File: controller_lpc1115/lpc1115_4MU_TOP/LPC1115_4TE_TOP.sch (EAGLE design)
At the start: 102 parts, among them P2 ISP, Q1 BC856, Q2 BCP52, Q3 BC847C, U1 LPC1115FBD48, U2 BD9G101, U3 XO32 12MHz

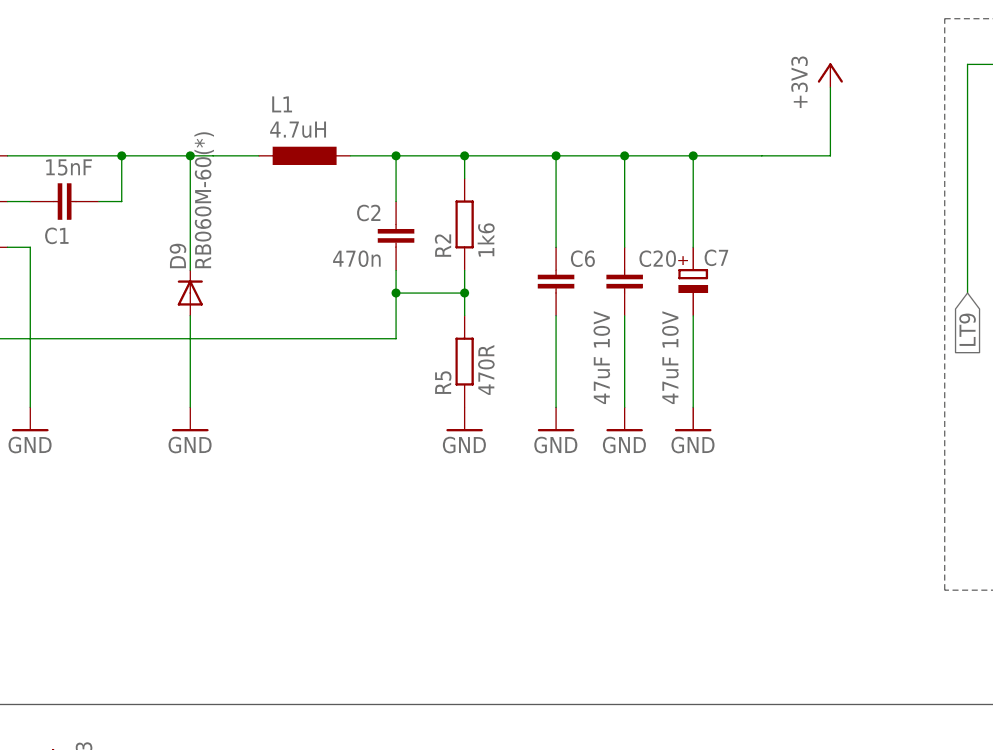
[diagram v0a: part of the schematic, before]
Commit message: [ctrl_4MU_TOP] - v2.0 alpha
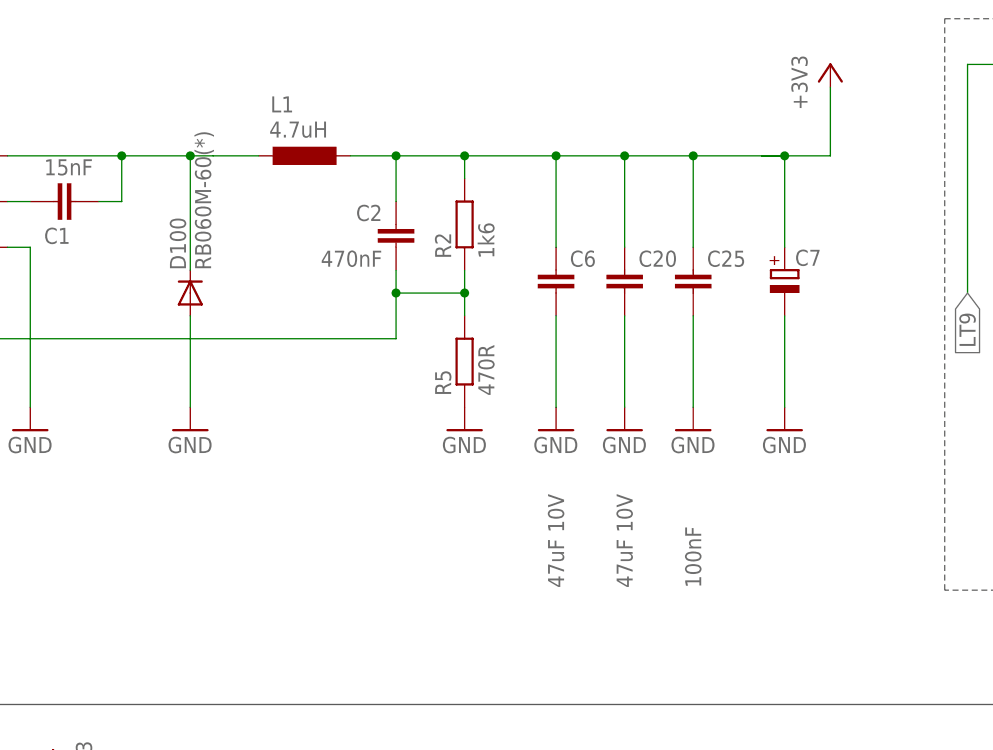
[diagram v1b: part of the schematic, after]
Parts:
- added C25: 100nF, rcl:C-EUC1206
- C2: value 470n -> 470nF
- C20, C6: device rcl:C-EUC1206 -> rcl:C-EUC0805
- renumbered D9 to D100
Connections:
- net +3V3: now also C25.1
- net GND: now also C25.2
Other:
- moved on the sheet: C7
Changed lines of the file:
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@@
 <part name="L1" library="rcl" library_urn="urn:adsk.eagle:library:334" deviceset="L-EU" device="L4532P" package3d_urn="urn:adsk.eagle:package:23484/1" value="4.7uH"/>
 <part name="C4" library="rcl" library_urn="urn:adsk.eagle:library:334" deviceset="C-EU" device="C0805" package3d_urn="urn:adsk.eagle:package:23617/2" value="4.7uF 50V"/>
-<part name="C6" library="rcl" library_urn="urn:adsk.eagle:library:334" deviceset="C-EU" device="C1206" package3d_urn="urn:adsk.eagle:package:23618/2" value="47uF 10V"/>
+<part name="C6" library="rcl" library_urn="urn:adsk.eagle:library:334" deviceset="C-EU" device="C0805" package3d_urn="urn:adsk.eagle:package:23617/2" value="47uF 10V"/>
 <part name="C1" library="rcl" library_urn="urn:adsk.eagle:library:334" deviceset="C-EU" device="C0805" package3d_urn="urn:adsk.eagle:package:23617/2" value="15nF"/>
 <part name="R2" library="rcl" library_urn="urn:adsk.eagle:library:334" deviceset="R-EU_" device="R0805" package3d_urn="urn:adsk.eagle:package:23553/2" value="1k6"/>
 <part name="R5" library="rcl" library_urn="urn:adsk.eagle:library:334" deviceset="R-EU_" device="R0805" package3d_urn="urn:adsk.eagle:package:23553/2" value="470R"/>
-<part name="C2" library="rcl" library_urn="urn:adsk.eagle:library:334" deviceset="C-EU" device="C0805" package3d_urn="urn:adsk.eagle:package:23617/2" value="470n"/>
-<part name="D9" library="diode" deviceset="DIODE-" device="SOD123" value="RB060M-60(*)"/>
+<part name="C2" library="rcl" library_urn="urn:adsk.eagle:library:334" deviceset="C-EU" device="C0805" package3d_urn="urn:adsk.eagle:package:23617/2" value="470nF"/>
+<part name="D100" library="diode" deviceset="DIODE-" device="SOD123" value="RB060M-60(*)"/>
 <part name="+3V35" library="supply1" deviceset="+3V3" device=""/>
 <part name="C13" library="rcl" library_urn="urn:adsk.eagle:library:334" deviceset="C-EU" device="C0805" package3d_urn="urn:adsk.eagle:package:23617/2" value="1uF"/>
@@
 <part name="D15" library="Diode_for_Selfbus-Projects" deviceset="DIODE-ZENER" device="SOD-123" package3d_urn="urn:adsk.eagle:package:40015434/2" value="DDZ9685"/>
 <part name="R1" library="rcl" library_urn="urn:adsk.eagle:library:334" deviceset="R-EU_" device="R2512" package3d_urn="urn:adsk.eagle:package:23545/2" value="24R  2512 1.0W"/>
-<part name="C20" library="rcl" library_urn="urn:adsk.eagle:library:334" deviceset="C-EU" device="C1206" package3d_urn="urn:adsk.eagle:package:23618/2" value="47uF 10V"/>
+<part name="C20" library="rcl" library_urn="urn:adsk.eagle:library:334" deviceset="C-EU" device="C0805" package3d_urn="urn:adsk.eagle:package:23617/2" value="47uF 10V"/>
 <part name="GND4" library="supply1" deviceset="GND" device=""/>
 <part name="C21" library="rcl" library_urn="urn:adsk.eagle:library:334" deviceset="C-EU" device="C0805" package3d_urn="urn:adsk.eagle:package:23617/2" value="100nF"/>
 <part name="C8" library="rcl" library_urn="urn:adsk.eagle:library:334" deviceset="C-EU" device="C0805" package3d_urn="urn:adsk.eagle:package:23617/2" value="100nF"/>
 <part name="C24" library="rcl" library_urn="urn:adsk.eagle:library:334" deviceset="C-EU" device="C0805" package3d_urn="urn:adsk.eagle:package:23617/2" value="1uF"/>
+<part name="C25" library="rcl" library_urn="urn:adsk.eagle:library:334" deviceset="C-EU" device="C1206" package3d_urn="urn:adsk.eagle:package:23618/2" value="100nF"/>
+<part name="GND7" library="supply1" deviceset="GND" device=""/>
 </parts>
 <sheets>
@@
 <instance part="C6" gate="G$1" x="200.66" y="226.06" smashed="yes">
 <attribute name="NAME" x="202.184" y="226.441" size="1.778" layer="95"/>
-<attribute name="VALUE" x="206.629" y="211.074" size="1.778" layer="96" rot="R90"/>
+<attribute name="VALUE" x="201.549" y="190.754" size="1.778" layer="96" rot="R90"/>
 </instance>
 <instance part="C1" gate="G$1" x="147.32" y="233.68" smashed="yes" rot="R270">
@@
 <attribute name="VALUE" x="181.356" y="226.441" size="1.778" layer="96" rot="MR0"/>
 </instance>
-<instance part="D9" gate="G$1" x="160.02" y="223.52" smashed="yes" rot="R90">
+<instance part="D100" gate="G$1" x="160.02" y="223.52" smashed="yes" rot="R90">
 <attribute name="NAME" x="159.5374" y="226.06" size="1.778" layer="95" rot="R90"/>
 <attribute name="VALUE" x="162.3314" y="226.06" size="1.778" layer="96" rot="R90"/>
@@
 <attribute name="SHEET" x="357.505" y="5.08" size="2.54" layer="94"/>
 </instance>
-<instance part="C7" gate="G$1" x="215.9" y="226.06" smashed="yes">
-<attribute name="NAME" x="217.043" y="226.5426" size="1.778" layer="95"/>
-</instance>
-<instance part="GND10" gate="1" x="215.9" y="208.28" smashed="yes">
-<attribute name="VALUE" x="213.36" y="205.74" size="1.778" layer="96"/>
+<instance part="C7" gate="G$1" x="226.06" y="226.06" smashed="yes">
+<attribute name="NAME" x="227.203" y="226.5426" size="1.778" layer="95"/>
+</instance>
+<instance part="GND10" gate="1" x="226.06" y="208.28" smashed="yes">
+<attribute name="VALUE" x="223.52" y="205.74" size="1.778" layer="96"/>
 </instance>
 <instance part="D16" gate="G$1" x="60.96" y="127" smashed="yes" rot="R90">
@@
 <instance part="C20" gate="G$1" x="208.28" y="226.06" smashed="yes">
 <attribute name="NAME" x="209.804" y="226.441" size="1.778" layer="95"/>
-<attribute name="VALUE" x="214.249" y="211.074" size="1.778" layer="96" rot="R90"/>
+<attribute name="VALUE" x="209.169" y="190.754" size="1.778" layer="96" rot="R90"/>
 </instance>
 <instance part="GND4" gate="1" x="208.28" y="208.28" smashed="yes">
@@
 <attribute name="NAME" x="301.244" y="91.821" size="1.778" layer="95"/>
 <attribute name="VALUE" x="301.244" y="86.741" size="1.778" layer="96"/>
+</instance>
+<instance part="C25" gate="G$1" x="215.9" y="226.06" smashed="yes">
+<attribute name="NAME" x="217.424" y="226.441" size="1.778" layer="95"/>
+<attribute name="VALUE" x="216.789" y="190.754" size="1.778" layer="96" rot="R90"/>
+</instance>
+<instance part="GND7" gate="1" x="215.9" y="208.28" smashed="yes">
+<attribute name="VALUE" x="213.36" y="205.74" size="1.778" layer="96"/>
 </instance>
 </instances>
@@
 </segment>
 <segment>
-<pinref part="D9" gate="G$1" pin="A"/>
+<pinref part="D100" gate="G$1" pin="A"/>
 <wire x1="160.02" y1="220.98" x2="160.02" y2="210.82" width="0.1524" layer="91"/>
 <pinref part="GND6" gate="1" pin="GND"/>
@@
 <pinref part="C7" gate="G$1" pin="-"/>
 <pinref part="GND10" gate="1" pin="GND"/>
-<wire x1="215.9" y1="220.98" x2="215.9" y2="210.82" width="0.1524" layer="91"/>
+<wire x1="226.06" y1="220.98" x2="226.06" y2="210.82" width="0.1524" layer="91"/>
 </segment>
 <segment>
@@
 <wire x1="208.28" y1="220.98" x2="208.28" y2="210.82" width="0.1524" layer="91"/>
 <pinref part="GND4" gate="1" pin="GND"/>
+</segment>
+<segment>
+<pinref part="C25" gate="G$1" pin="2"/>
+<wire x1="215.9" y1="220.98" x2="215.9" y2="210.82" width="0.1524" layer="91"/>
+<pinref part="GND7" gate="1" pin="GND"/>
 </segment>
 </net>
@@
 <wire x1="152.4" y1="233.68" x2="152.4" y2="238.76" width="0.1524" layer="91"/>
 <pinref part="L1" gate="G$1" pin="1"/>
-<pinref part="D9" gate="G$1" pin="C"/>
+<pinref part="D100" gate="G$1" pin="C"/>
 <wire x1="160.02" y1="226.06" x2="160.02" y2="238.76" width="0.1524" layer="91"/>
 <junction x="152.4" y="238.76"/>
@@
 <wire x1="200.66" y1="238.76" x2="208.28" y2="238.76" width="0.1524" layer="91"/>
 <wire x1="208.28" y1="238.76" x2="215.9" y2="238.76" width="0.1524" layer="91"/>
-<wire x1="215.9" y1="238.76" x2="223.52" y2="238.76" width="0.1524" layer="91"/>
+<wire x1="215.9" y1="238.76" x2="226.06" y2="238.76" width="0.1524" layer="91"/>
+<wire x1="226.06" y1="238.76" x2="223.52" y2="238.76" width="0.1524" layer="91"/>
 <wire x1="223.52" y1="238.76" x2="231.14" y2="238.76" width="0.1524" layer="91"/>
 <wire x1="190.5" y1="236.22" x2="190.5" y2="238.76" width="0.1524" layer="91"/>
@@
 <junction x="200.66" y="238.76"/>
 <pinref part="C7" gate="G$1" pin="+"/>
-<wire x1="215.9" y1="238.76" x2="215.9" y2="228.6" width="0.1524" layer="91"/>
-<junction x="215.9" y="238.76"/>
+<wire x1="226.06" y1="238.76" x2="226.06" y2="228.6" width="0.1524" layer="91"/>
+<junction x="226.06" y="238.76"/>
 <pinref part="C20" gate="G$1" pin="1"/>
 <wire x1="208.28" y1="228.6" x2="208.28" y2="238.76" width="0.1524" layer="91"/>
 <junction x="208.28" y="238.76"/>
-</segment>
-<segment>
+<pinref part="C25" gate="G$1" pin="1"/>
+<wire x1="215.9" y1="228.6" x2="215.9" y2="238.76" width="0.1524" layer="91"/>
+<junction x="215.9" y="238.76"/>
+</segment>
+<segment>
